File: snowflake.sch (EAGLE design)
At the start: 28 parts, among them U1 ATTINY13A-PU

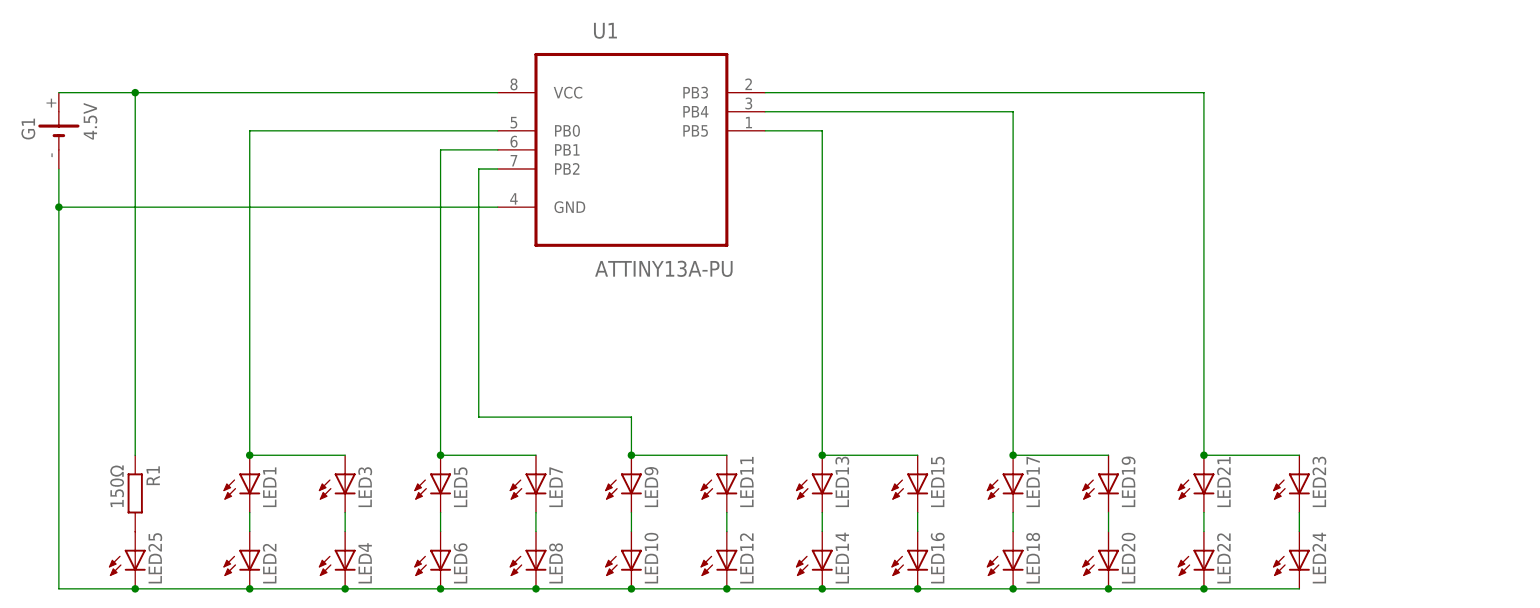
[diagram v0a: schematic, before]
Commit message: v1.0
That’s it. (I’m pretty sure)
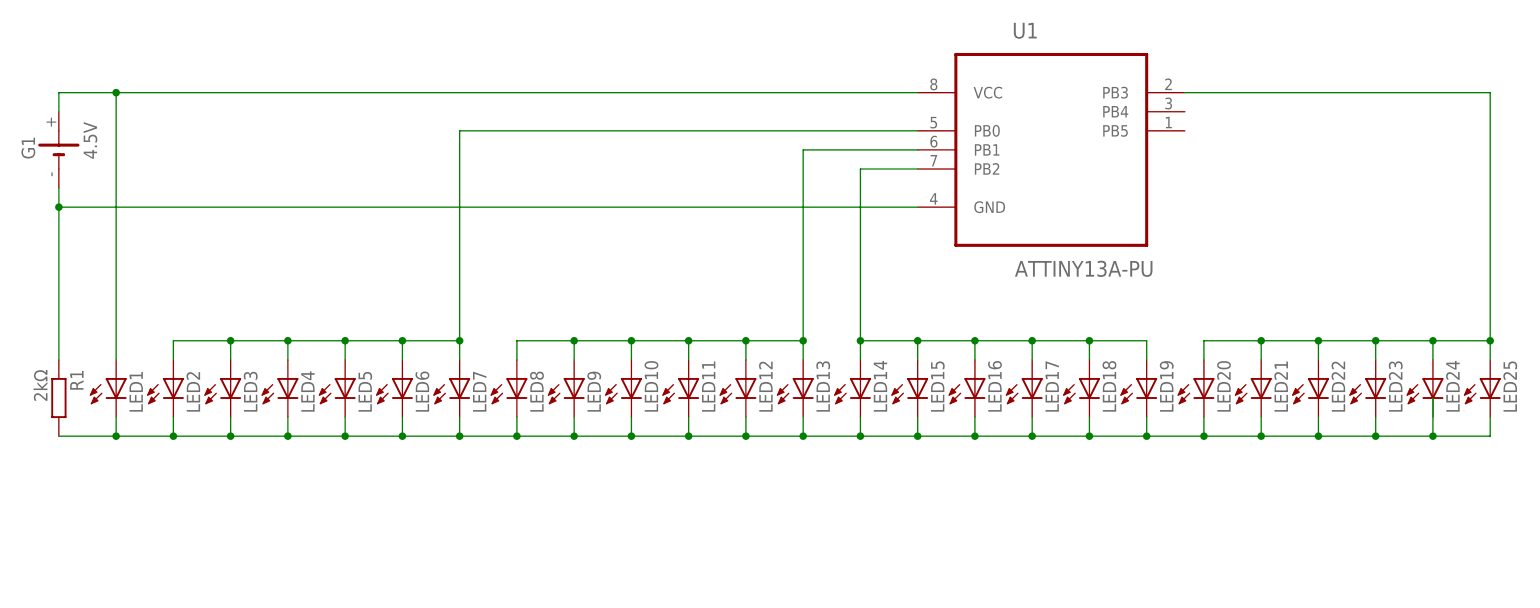
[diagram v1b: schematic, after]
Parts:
- R1: value 150Ω -> 2kΩ
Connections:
- removed net N$10: LED19.C, LED20.A
- removed net N$11: LED21.C, LED22.A
- removed net N$12: LED23.C, LED24.A
- removed net N$13: LED25.A, R1.2
- removed net N$14: G1.-, LED10.C, LED12.C, LED14.C, LED16.C, LED18.C, LED2.C, LED20.C, LED22.C, LED24.C, LED25.C, LED4.C, LED6.C, LED8.C, U1.GND
- removed net N$16: LED1.A, LED3.A, U1.PB0
- removed net N$17: LED5.A, LED7.A, U1.PB1
- removed net N$19: LED13.A, LED15.A, U1.PB5
- removed net N$20: LED21.A, LED23.A, U1.PB3
- removed net N$21: LED17.A, LED19.A, U1.PB4
- removed net N$6: LED11.C, LED12.A
- removed net N$7: LED13.C, LED14.A
- removed net N$8: LED15.C, LED16.A
- removed net N$9: LED17.C, LED18.A
- net N$1: now also LED10.C, LED11.C, LED12.C, LED13.C, LED14.C, LED15.C, LED16.C, LED17.C, LED18.C, LED19.C, LED2.C, LED20.C, LED21.C, LED22.C, LED23.C, LED25.C, LED3.C, LED4.C, LED5.C, LED6.C, LED7.C, LED8.C, LED9.C, R1.2; no longer LED2.A
- net N$15: now also LED1.A; no longer R1.1
- net N$18: now also G1.-, R1.1, U1.GND; no longer LED11.A, LED9.A, U1.PB2
- net N$2: now also LED14.A, LED15.A, LED16.A, LED17.A, LED18.A, LED19.A, U1.PB2; no longer LED3.C, LED4.A
- net N$3: now also LED10.A, LED11.A, LED12.A, LED13.A, LED8.A, LED9.A, U1.PB1; no longer LED5.C, LED6.A
- net N$4: now also LED2.A, LED3.A, LED4.A, LED5.A, LED6.A, LED7.A, U1.PB0; no longer LED7.C, LED8.A
- net N$5: now also LED20.A, LED21.A, LED22.A, LED23.A, LED24.A, LED25.A, U1.PB3; no longer LED10.A, LED9.C
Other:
- moved on the sheet: G1, LED1, LED10, LED11, LED12, LED13, LED14, LED15, LED16, LED17, LED18, LED19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
